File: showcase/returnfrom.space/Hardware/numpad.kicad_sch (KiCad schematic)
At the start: 59 parts, among them J21 Conn_01x08_Socket, J22 USB_C_Receptacle_USB2.0_16P, SW1 SW_SPST, SW10 SW_SPST, SW11 SW_SPST, SW12 SW_SPST, SW13 SW_SPST, SW14 SW_SPST, SW15 SW_SPST, SW16 SW_SPST, SW17 RESET, SW18 BOOTSEL, SW2 SW_SPST, SW3 SW_SPST, SW4 SW_SPST, SW5 SW_SPST, SW6 SW_SPST, SW7 SW_SPST, SW8 SW_SPST, SW9 SW_SPST, U3 RP2040, U8 W25Q128JVS

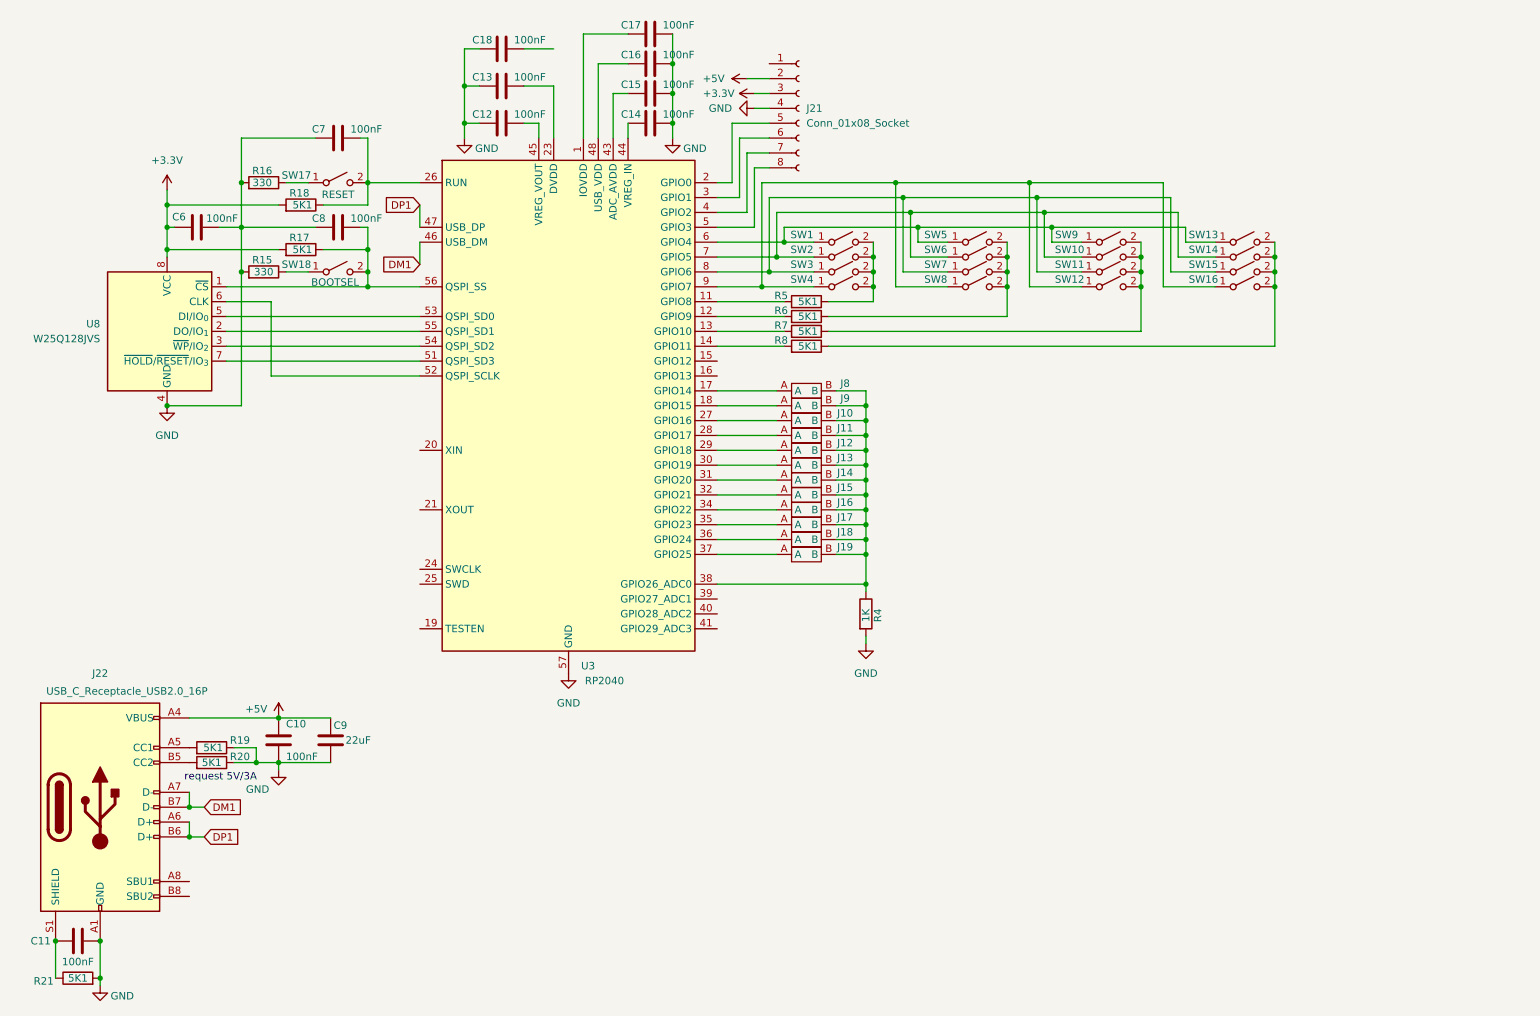
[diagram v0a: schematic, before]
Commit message: updated
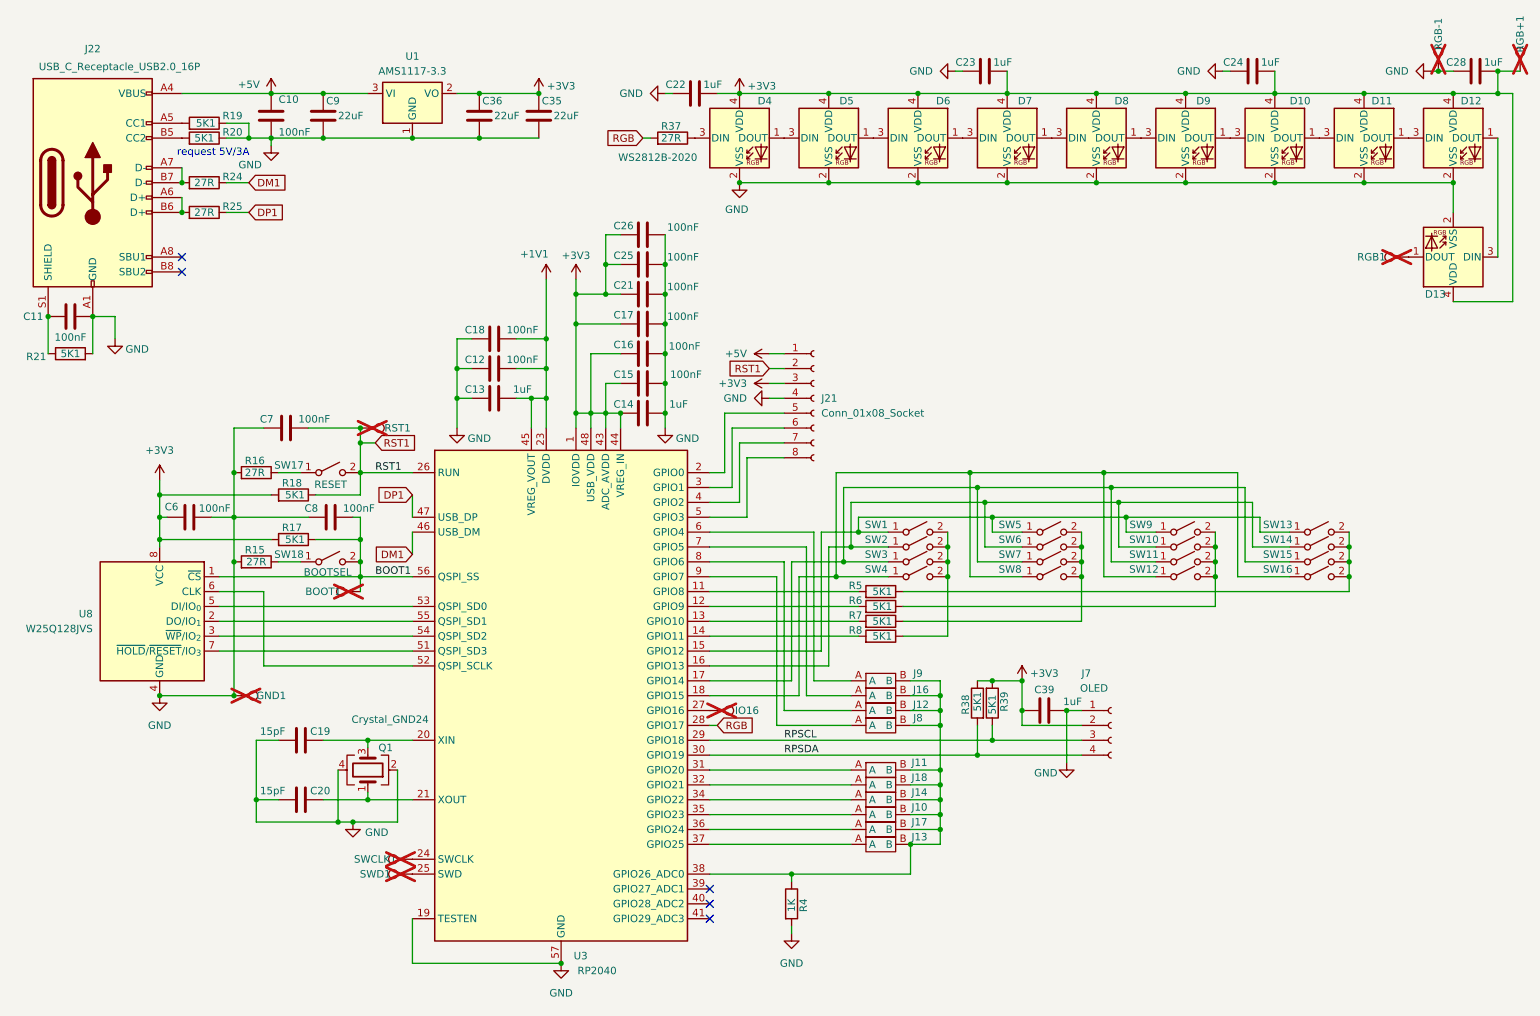
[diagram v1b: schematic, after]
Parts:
- removed J15, J19: ~, spacescape:Untitled, symbol spacescape:RES-PAD
- added BOOT1, GND1, IO16, RGB+1, RGB-1, RGB1, RST1, SWCLK1, SWD1: TestPoint, TestPoint:TestPoint_Pad_D2.0mm, symbol Connector:TestPoint
- added C19, C20: 15pF, Capacitor_SMD:C_0402_1005Metric, symbol Device:C
- added C21, C25, C26: 100nF, Capacitor_SMD:C_0402_1005Metric, symbol Device:C
- added C22, C23, C24, C28, C39: 1uF, Capacitor_SMD:C_0402_1005Metric, symbol Device:C
- added C35, C36: 22uF, Capacitor_SMD:C_0805_2012Metric, symbol Device:C
- added D10, D11, D12, D13, D4, D5, D6, D7, D8, D9: WS2812B-2020, LED_SMD:LED_WS2812B-2020_PLCC4_2.0x2.0mm, symbol LED:WS2812B-2020
- added J7: OLED, TG9541:Display_128x64_096_I2C, symbol Connector:Conn_01x04_Socket
- added Q1: Crystal_GND24, Crystal:Crystal_SMD_3225-4Pin_3.2x2.5mm, symbol Device:Crystal_GND24
- added R24, R25, R37: 27R, Resistor_SMD:R_0402_1005Metric, symbol Device:R
- added R38, R39: 5K1, Resistor_SMD:R_0402_1005Metric, symbol Device:R
- added U1: AMS1117-3.3, Package_TO_SOT_SMD:SOT-223-3_TabPin2, symbol Regulator_Linear:AMS1117-3.3
- C13: renamed from C12; value 100nF -> 1uF
- C14: value 100nF -> 1uF
- R15, R16: value 330 -> 27R
- renumbered C13 to C12
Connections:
- net +3.3V is gone; now on net +3V3: C6.1, J21.3 (Pin_3), R17.2, R18.2, U8.8 (VCC)
- net +5V: now also J21.1 (Pin_1), U1.3 (VI); no longer J21.2 (Pin_2)
- net DM1: now also R24.1; no longer J22.A7 (D-), J22.B7 (D-)
- net DP1: now also R25.1; no longer J22.A6 (D+), J22.B6 (D+)
- net GND: now also U3.19 (TESTEN), C19.2, C20.2, C21.2, C22.1, C23.1, C24.1, C25.2, C26.2, C28.1, C35.2, C36.2, C39.2, D10.2 (VSS), D11.2 (VSS), D12.2 (VSS), D13.2 (VSS), D4.2 (VSS), D5.2 (VSS), D6.2 (VSS), D7.2 (VSS), D8.2 (VSS), D9.2 (VSS), GND1.1, J7.1 (Pin_1), Q1.2, Q1.4, RGB-1.1, U1.1 (GND)
- net at SW10.1 (A), SW14.1 (A), SW2.1 (A)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: now also U3.16 (GPIO13); no longer U3.7 (GPIO5)
- net at SW13.2 (B), SW14.2 (B), SW15.2 (B)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: now also R5.1; no longer R8.1
- net at SW1.1 (A), SW13.1 (A), SW5.1 (A)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: now also U3.15 (GPIO12); no longer U3.6 (GPIO4)
- net at SW5.2 (B), SW6.2 (B), SW7.2 (B)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: now also R7.1; no longer R6.1
- net at SW11.1 (A), SW15.1 (A), SW3.1 (A)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: now also U3.17 (GPIO14); no longer U3.8 (GPIO6)
- net at J12.A: now also U3.8 (GPIO6); no longer U3.29 (GPIO18)
- net at J14.A: now also U3.34 (GPIO22); no longer U3.31 (GPIO20)
- net at J13.A: now also U3.37 (GPIO25); no longer U3.30 (GPIO19)
- net at J16.A: now also U3.7 (GPIO5); no longer U3.34 (GPIO22)
- net at SW12.1 (A), SW16.1 (A), SW4.1 (A)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: now also U3.18 (GPIO15); no longer U3.9 (GPIO7)
- net +1V1: now reaches C12.2, U3.23 (DVDD), U3.50 (DVDD)
- net +1V1: now also C13.2, C18.2, U3.45 (VREG_VOUT)
- net +3V3: now reaches C17.1, U3.1 (IOVDD), U3.10 (IOVDD), U3.22 (IOVDD), U3.33 (IOVDD), U3.42 (IOVDD), U3.49 (IOVDD)
- net +3V3: now also C14.1, C15.1, C16.1, U3.43 (ADC_AVDD), U3.44 (VREG_IN), U3.48 (USB_VDD), C21.1, C22.2, C23.2, C24.2, C25.1, C26.1, C28.2, C35.1, C36.1, C39.1, D10.4 (VDD), D11.4 (VDD), D12.4 (VDD), D13.4 (VDD), D4.4 (VDD), D5.4 (VDD), D6.4 (VDD), D7.4 (VDD), D8.4 (VDD), D9.4 (VDD), J7.2 (Pin_2), R38.1, R39.2, RGB+1.1, U1.2 (VO)
- net at J8.A: now also U3.9 (GPIO7); no longer U3.17 (GPIO14)
- net at J9.A: now also U3.6 (GPIO4); no longer U3.18 (GPIO15)
- net at U3.20 (XIN): now also C19.1, Q1.3
- net at U3.21 (XOUT): now also C20.1, Q1.1
- net at U3.24 (SWCLK): now also SWCLK1.1
- net at U3.25 (SWD): now also SWD1.1
- net RST1: now reaches C7.2, R18.1, SW17.2 (B), U3.26 (RUN)
- net RST1: now also J21.2 (Pin_2), RST1.1
- net at U3.27 (GPIO16): now also IO16.1; no longer J10.A
- net at J11.A: now also U3.31 (GPIO20); no longer U3.28 (GPIO17)
- net at U3.32 (GPIO21): now also J18.A
- net at U3.35 (GPIO23): now also J10.A; no longer J17.A
- net at U3.36 (GPIO24): now also J17.A; no longer J18.A
- net BOOT1: now reaches C8.2, R17.1, SW18.2 (B), U3.56 (QSPI_SS), U8.1 (~{CS})
- net BOOT1: now also BOOT1.1
- net at SW1.2 (B), SW2.2 (B), SW3.2 (B)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: now also R8.1; no longer R5.1
- net at SW10.2 (B), SW11.2 (B), SW12.2 (B)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: now also R6.1; no longer R7.1
- new net: D8.1 (DOUT), D9.3 (DIN)
- new net: D7.1 (DOUT), D8.3 (DIN)
- new net: D5.1 (DOUT), D6.3 (DIN)
- new net: D4.1 (DOUT), D5.3 (DIN)
- new net: D4.3 (DIN), R37.1
- new net: D13.1 (DOUT), RGB1.1
- new net: D6.1 (DOUT), D7.3 (DIN)
- new net: J22.A6 (D+), J22.B6 (D+), R25.2
- new net: J22.A7 (D-), J22.B7 (D-), R24.2
- new net: D12.1 (DOUT), D13.3 (DIN)
- new net: D11.1 (DOUT), D12.3 (DIN)
- new net: D10.3 (DIN), D9.1 (DOUT)
- new net: D10.1 (DOUT), D11.3 (DIN)
- new net RGB: R37.2, U3.28 (GPIO17)
- new net RPSCL: J7.3 (Pin_3), R39.1, U3.29 (GPIO18)
- new net RPSDA: J7.4 (Pin_4), R38.2, U3.30 (GPIO19)
- no-connect marks 0 -> 5
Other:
- moved on the sheet: C10, C11, C12, C13, C14, C15, C16, C17, C18, C6, C7, C8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
